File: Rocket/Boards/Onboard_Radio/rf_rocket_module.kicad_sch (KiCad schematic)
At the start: 12 parts

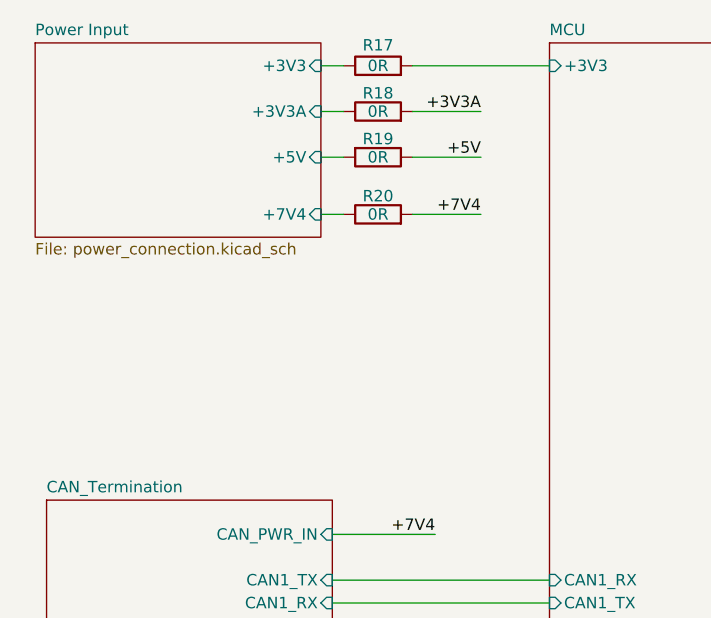
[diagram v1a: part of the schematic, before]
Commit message: updates
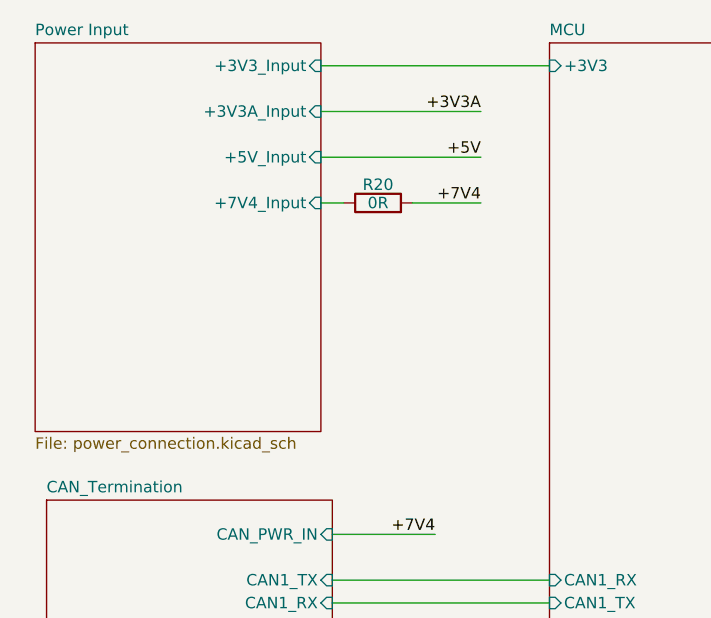
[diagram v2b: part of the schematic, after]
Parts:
- removed R17, R18, R19: 0R, Resistor_SMD:R_0603_1608Metric, symbol Device:R
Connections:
- net Power Input/+7V4 renamed Power Input/+7V4_Input
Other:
- sheet Power Input ports: added +3V3A_Input, +3V3_Input, +5V_Input, +7V4_Input; removed +3V3, +3V3A, +5V, +7V4
- moved on the sheet: R20
